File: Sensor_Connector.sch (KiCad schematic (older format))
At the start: 9 parts, among them J3 Sensor_Conn

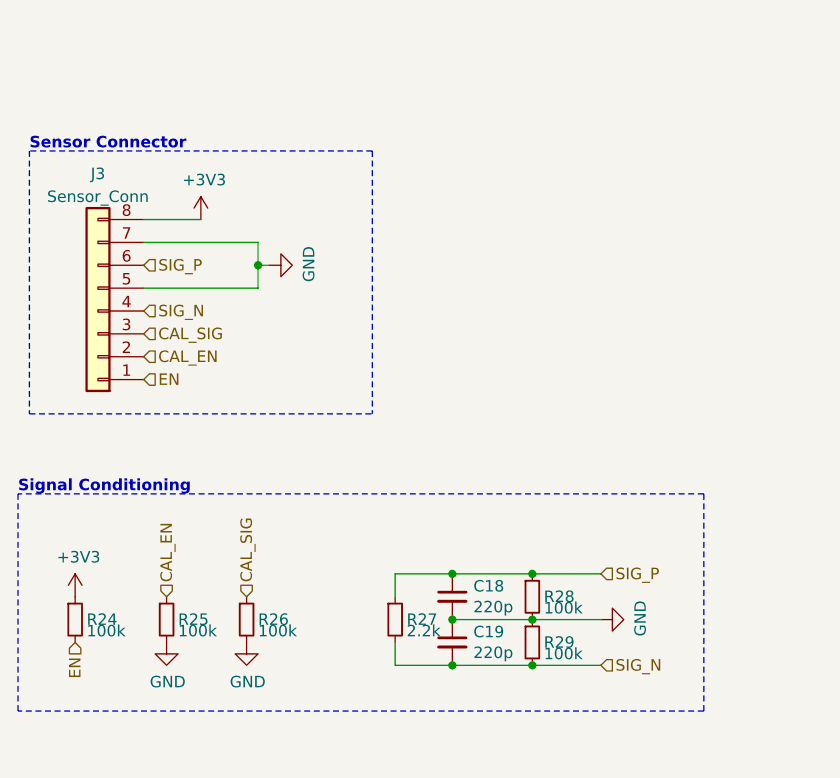
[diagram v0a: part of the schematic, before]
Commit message: PCB Layout Checkpoint
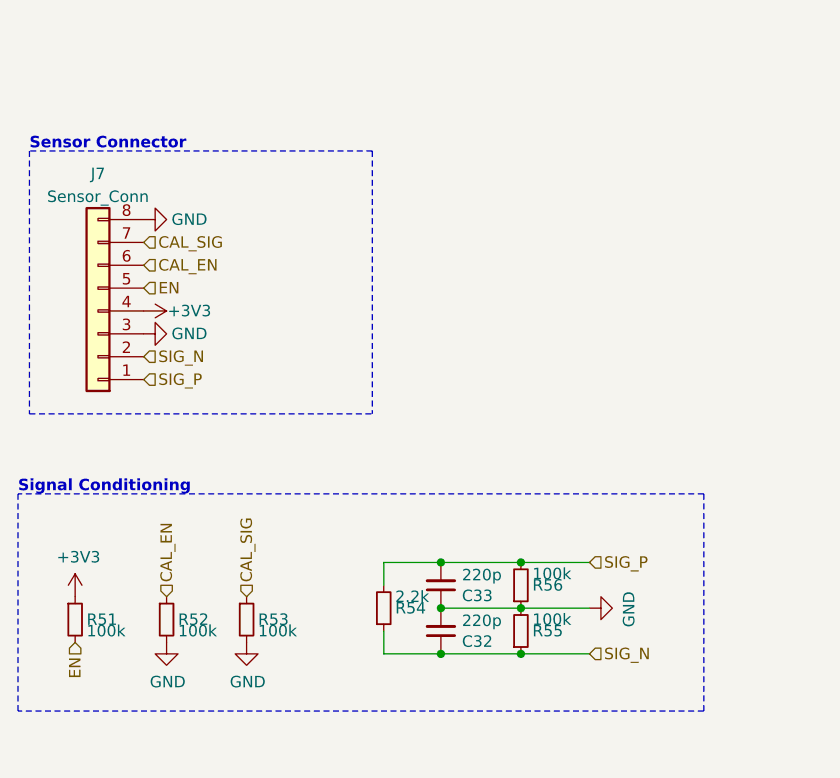
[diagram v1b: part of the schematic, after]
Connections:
- net +3V3: now also J3.4 (Pin_4); no longer J3.8 (Pin_8)
- net CAL_EN: now also J3.6 (Pin_6); no longer J3.2 (Pin_2)
- net CAL_SIG: now also J3.7 (Pin_7); no longer J3.3 (Pin_3)
- net EN: now also J3.5 (Pin_5); no longer J3.1 (Pin_1)
- net GND: now also J3.3 (Pin_3), J3.8 (Pin_8); no longer J3.5 (Pin_5), J3.7 (Pin_7)
- net SIG_N: now also C18.1, J3.2 (Pin_2), R27.1, R28.1; no longer C19.2, J3.4 (Pin_4), R27.2, R29.2
- net SIG_P: now also C19.2, J3.1 (Pin_1), R27.2, R29.2; no longer C18.1, J3.6 (Pin_6), R27.1, R28.1
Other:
- moved on the sheet: C32, C33, R54, R55, R56

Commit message: Major Commit with Final PCB Design
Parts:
- removed R24, R25, R26: 100k, Resistor_SMD:R_0603_1608Metric_Pad1.05x0.95mm_HandSolder, symbol Device:R_Small
- J3: footprint Connector_PinHeader_2.54mm:PinHeader_1x08_P2.54mm_Vertical -> Connector_PinHeader_2.00mm:PinHeader_2x04_P2.00mm_Vertical; symbol Connector_Generic:Conn_01x08 -> Connector_Generic:Conn_02x04_Odd_Even
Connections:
- net +3V3: now also J3.1 (Pin_1); no longer J3.4 (Pin_4)
- net CAL_EN: now also J3.8 (Pin_8); no longer J3.6 (Pin_6)
- net EN: now also J3.6 (Pin_6); no longer J3.5 (Pin_5)
- net GND: now also J3.5 (Pin_5); no longer J3.8 (Pin_8)
- net SIG_N: now also J3.4 (Pin_4); no longer J3.2 (Pin_2)
- net SIG_P: now also J3.2 (Pin_2); no longer J3.1 (Pin_1)
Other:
- moved on the sheet: J7
